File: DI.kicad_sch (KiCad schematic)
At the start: 50 parts, among them J10 Screw_Terminal_01x02, J11 Screw_Terminal_01x02, J12 Screw_Terminal_01x02, J9 Screw_Terminal_01x02, U18 CNY173SR2VM, U19 CNY173SR2VM, U20 CNY173SR2VM, U21 CNY173SR2VM, U22 MM74HC14M

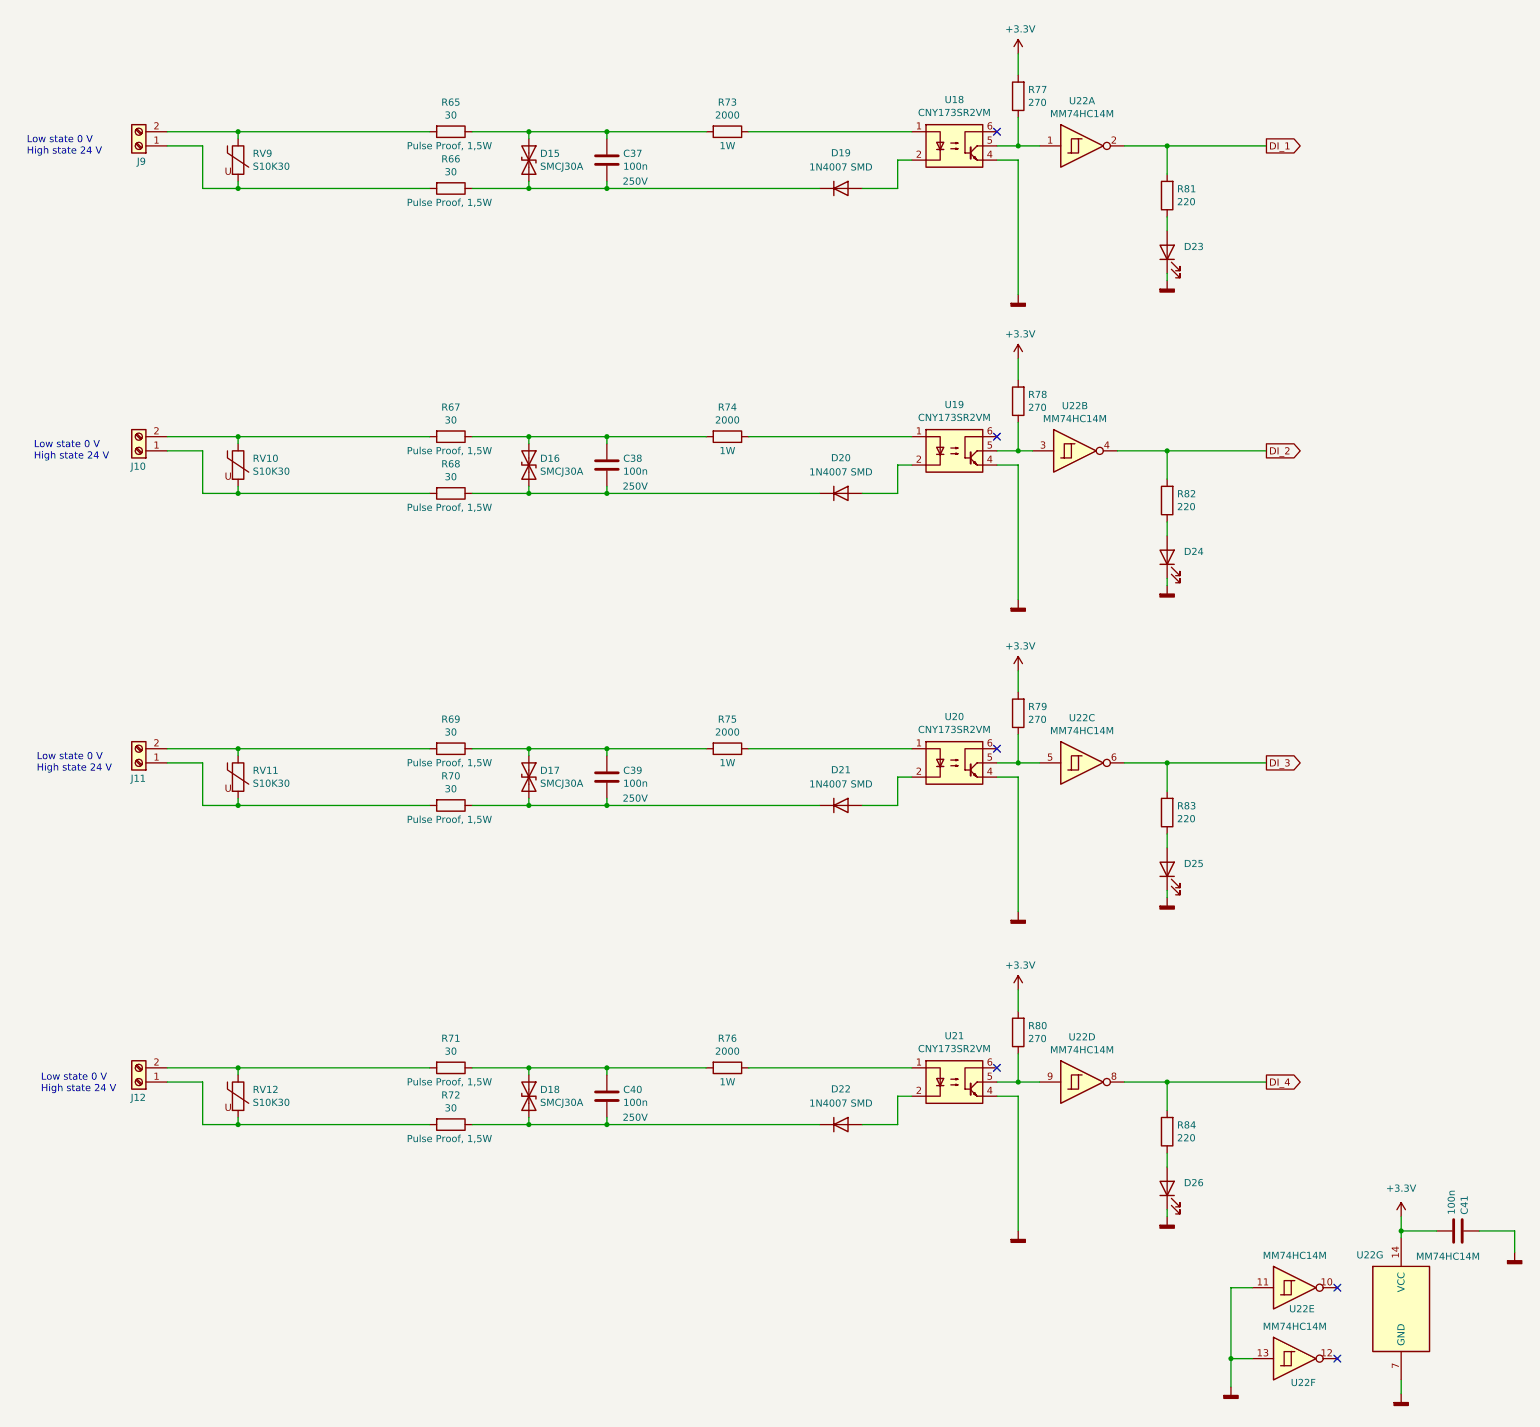
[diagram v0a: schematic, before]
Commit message: alueet laatikoitu, ensimmäiset input osat laitettu
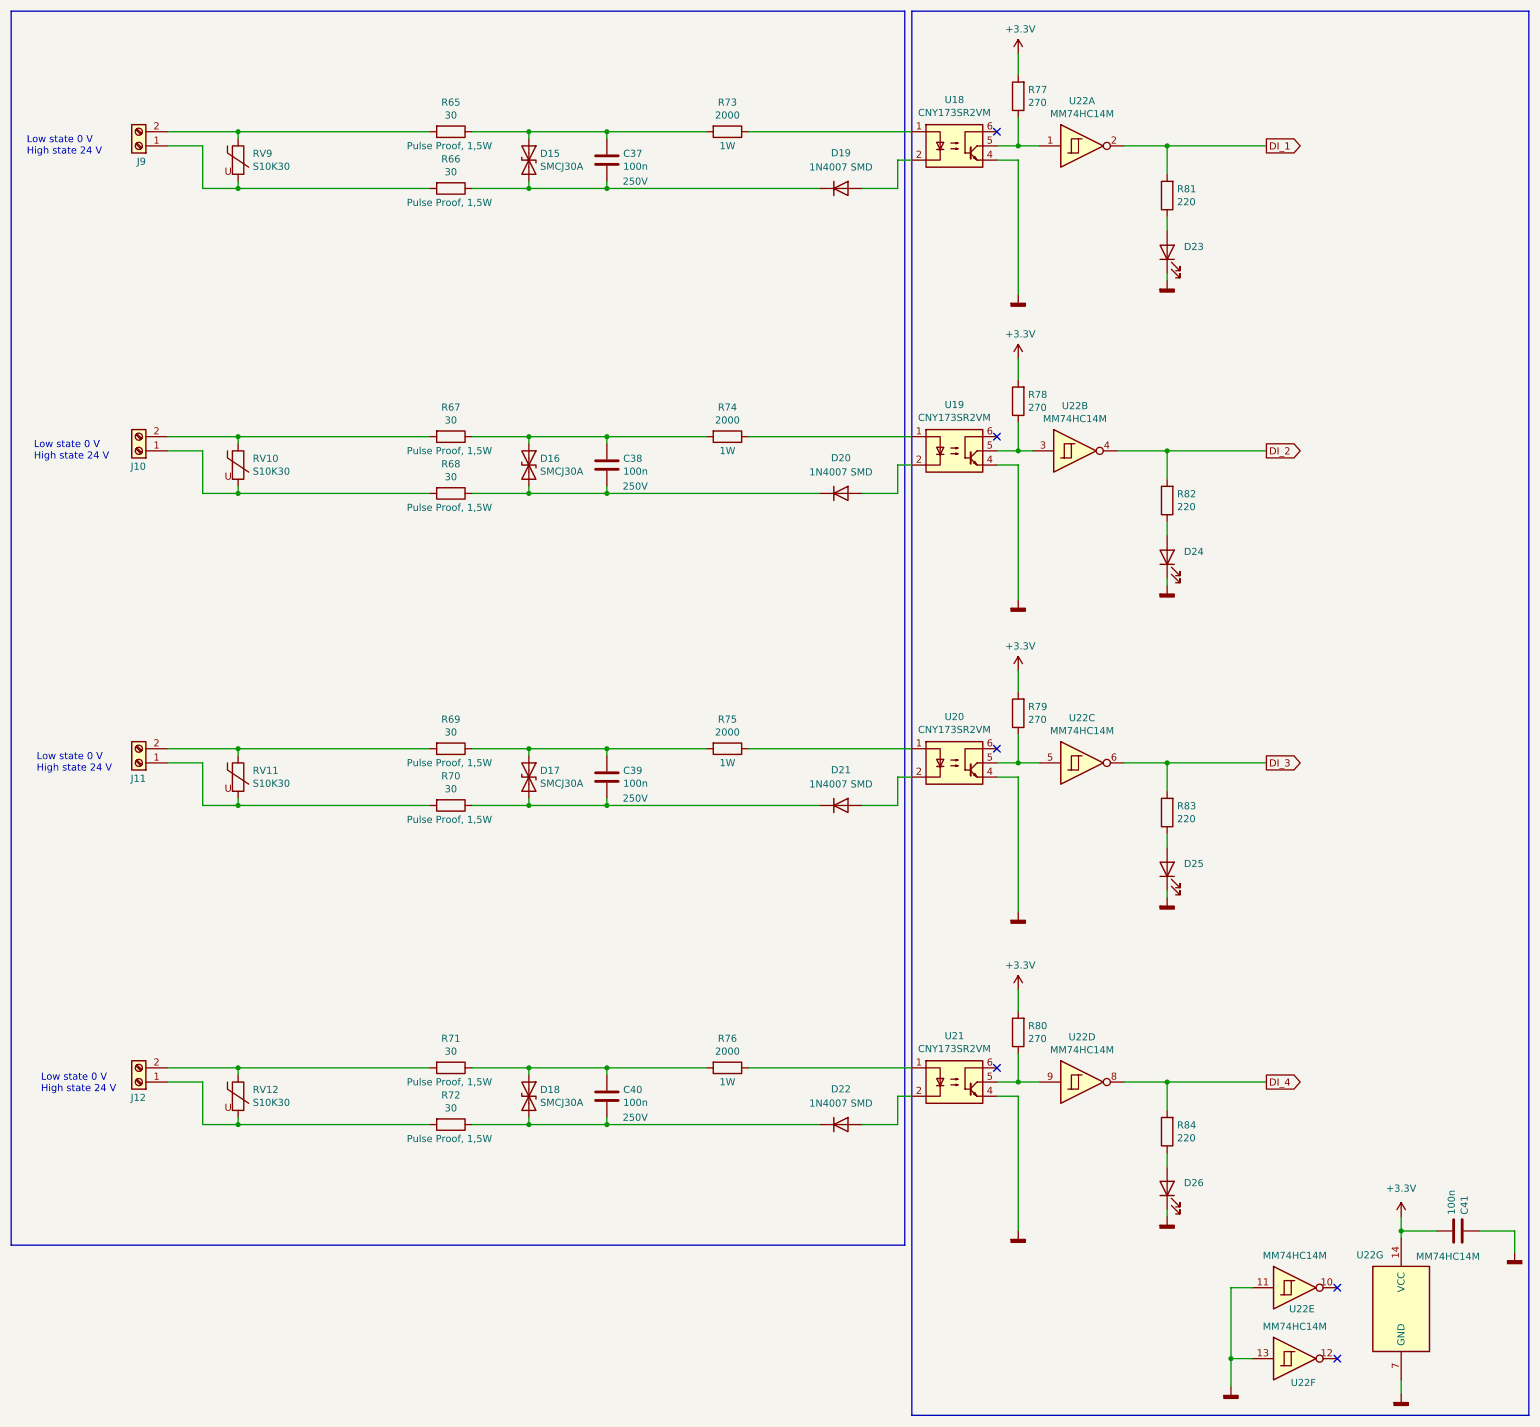
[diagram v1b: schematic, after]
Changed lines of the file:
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@@
 	(generator_version "9.0")
 	(paper "A3")
+	(rectangle
+		(start 200.66 22.86)
+		(end 311.15 274.32)
+		(stroke
+			(width 0)
+			(type default)
+			(color 244 0 255 1)
+		)
+		(fill
+			(type none)
+		)
+	)
+	(rectangle
+		(start 39.37 22.86)
+		(end 199.39 243.84)
+		(stroke
+			(width 0)
+			(type default)
+			(color 244 0 255 1)
+		)
+		(fill
+			(type none)
+		)
+	)
 	(text "Low state 0 V\nHigh state 24 V\n"
 		(exclude_from_sim no)
